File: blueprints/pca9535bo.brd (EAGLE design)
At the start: 28.3 x 18.1 mm, 9 parts, among them IC1 PCA9535D, J1 0R, J2 0R, J3 0R

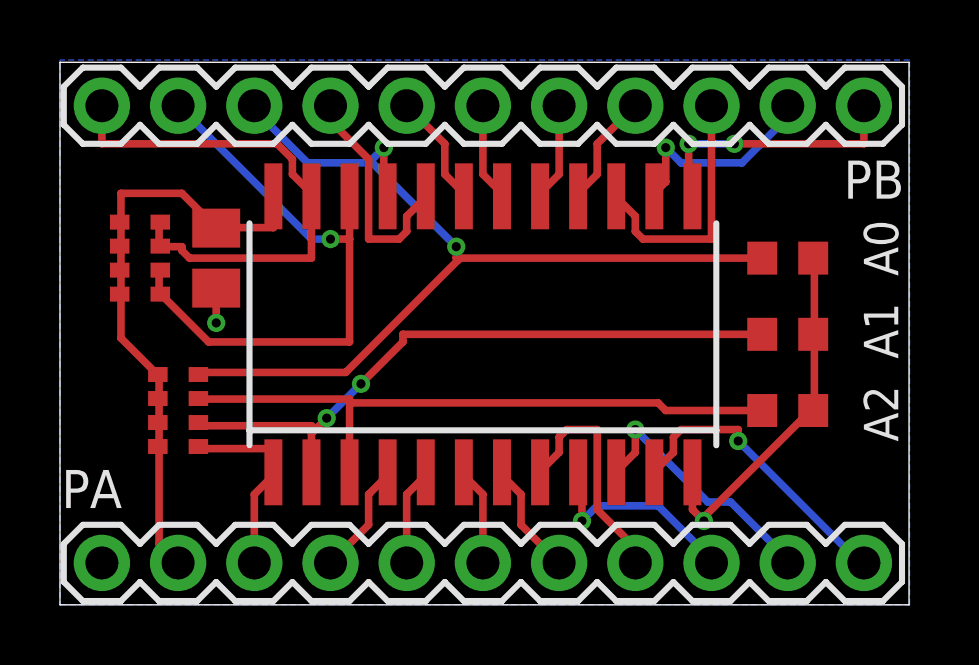
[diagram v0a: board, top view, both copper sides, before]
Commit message: cleaned up
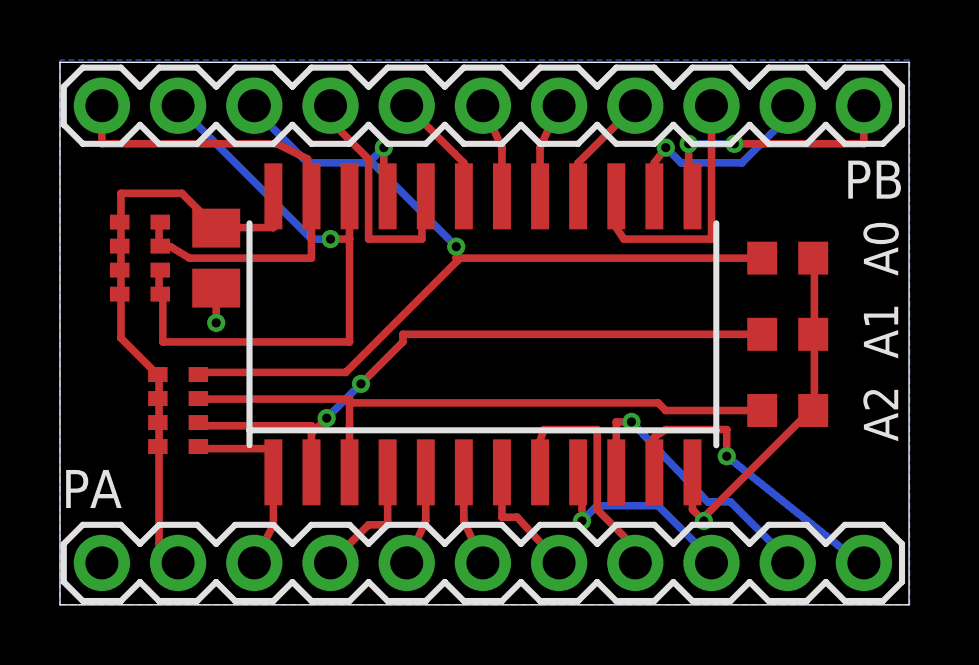
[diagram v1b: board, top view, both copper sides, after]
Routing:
- net SCL: track 20.2 -> 21.1 mm
- net PA6: track 8.68 -> 9.45 mm
